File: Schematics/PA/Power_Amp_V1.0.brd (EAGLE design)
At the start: 46.7 x 73.3 mm, 99 parts, among them J1 4_PIN_AMPCONN, J11 SCREW_TERMINAL_4, J12 1725724, J13 1725724, J14 1725724, U1 LME49830, U2 LME49830, U3 LME49830

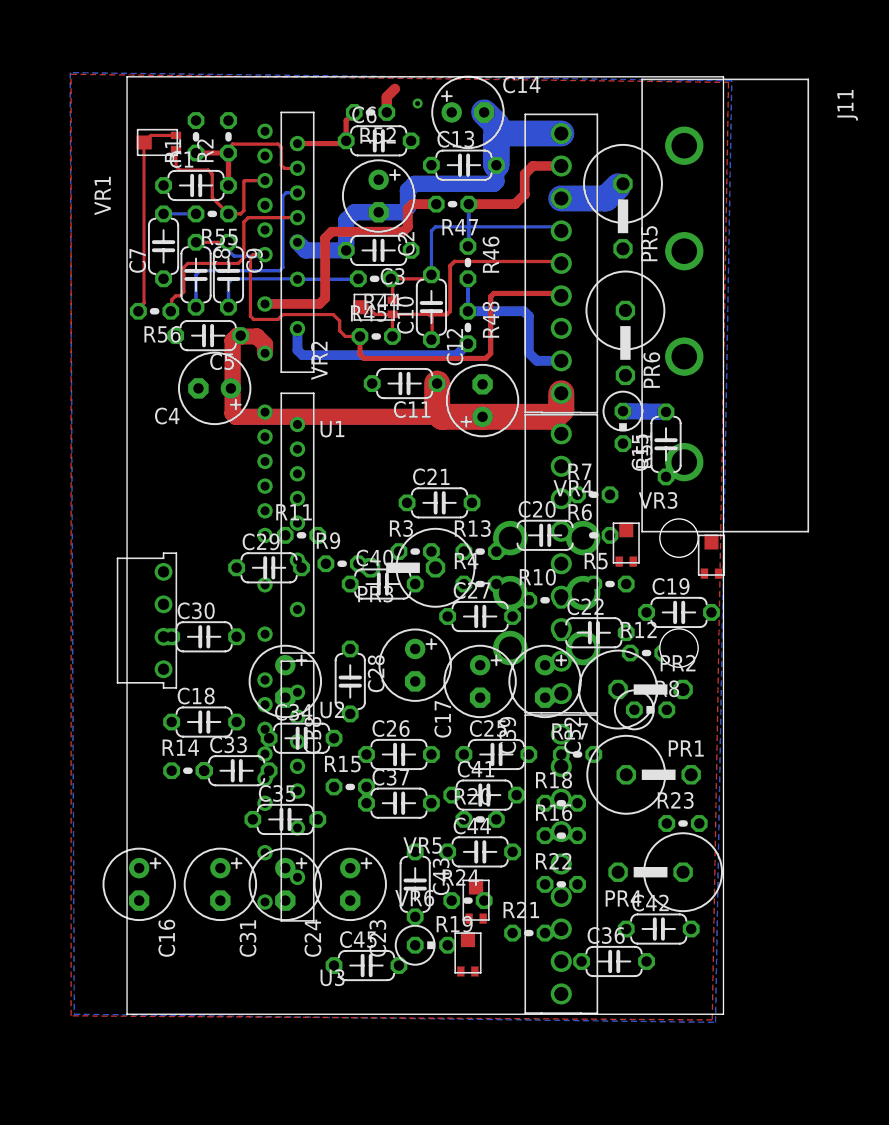
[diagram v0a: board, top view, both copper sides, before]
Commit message: Finished My PA and made changes to Carlos' PA
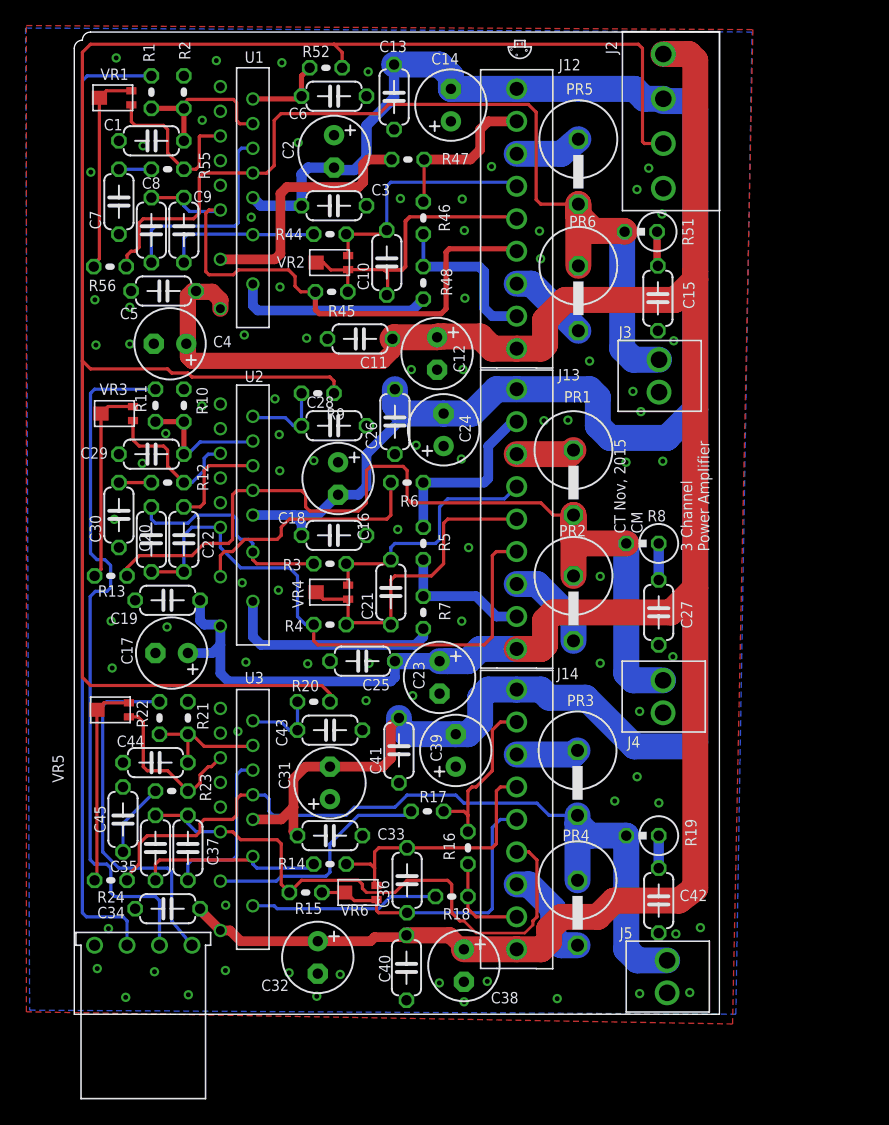
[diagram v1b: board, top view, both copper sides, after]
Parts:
- removed J11: SCREW_TERMINAL_4, Amplifier_Parts:SCREW_TERMINAL_4
- added J2: 1984633, Amplifier_Parts:1984633
- added J3, J4, J5: 2TERMINAL_SPEAKER, Amplifier_Parts:2TERMINAL_SPEAKER
- U$17: value MOLEX_6P -> (none); device Amplifier_Parts:MOLEX_6P -> PersonalLogos:MUSHROOM
- moved VR3 47.7 mm to (3.49, 47.0), turned to 90 degrees
- moved U$17 45.2 mm to (34.9, 75.4), turned to 180 degrees
- moved R23 40.1 mm to (7.62, 17.5), turned to 180 degrees
- moved C19 40.0 mm to (7.30, 32.4), turned to 180 degrees
- moved R12 39.8 mm to (7.30, 41.6), turned to 180 degrees
- moved C24 37.7 mm to (28.9, 45.7), turned to 90 degrees
- moved C16 35.4 mm to (20.6, 41.9)
- moved R22 34.0 mm to (6.67, 23.2), turned to 90 degrees
- moved C22 32.9 mm to (8.57, 37.1), turned to 90 degrees
- moved R10 32.1 mm to (8.57, 47.6), turned to 90 degrees
- moved VR5 32.1 mm to (3.17, 23.8), turned to 90 degrees
- moved R21 31.5 mm to (8.89, 23.2), turned to 90 degrees
- moved C20 30.8 mm to (6.03, 37.1), turned to 90 degrees
- moved C40 30.1 mm to (26.0, 3.64), turned to 270 degrees
- moved R13 29.0 mm to (2.86, 34.3), turned to 180 degrees
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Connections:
- net BASS renamed N$1
- net GND: now also J2.P$1, J3.P$2, J4.P$2, J5.P$2; no longer J11.1, U$17.P$2, U$17.P$4, U$17.P$6
- net MUTE: now also J2.P$2; no longer J11.2
- net N$12: now also J4.P$1; no longer U$17.P$3
- net N$75: now also J3.P$1; no longer U$17.P$1
- net N$77: now also J5.P$1; no longer U$17.P$5
- net V+: now also J2.P$4; no longer J11.4
- net V-: now also J2.P$3; no longer J11.3
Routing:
- net V+: track 42.0 -> 243.7 mm
- net V-: track 33.4 -> 195.3 mm
- net MUTE: track 2.10 -> 146.0 mm
- net RIGHT: track 0.00 -> 76.3 mm
- net N$12: track 0.00 -> 71.4 mm
- net N$75: track 16.2 -> 81.5 mm
- net N$77: track 0.00 -> 64.5 mm
- net N$1: track 0.00 -> 55.3 mm
- net L_VBE_E: track 0.00 -> 46.0 mm
- net B_VBE_E: track 0.00 -> 45.8 mm
- net LEFT: track 0.00 -> 28.4 mm
- net B_VBE_B: track 0.00 -> 25.4 mm
- net L_VBE_B: track 0.00 -> 23.2 mm
- net L_VBE_C: track 0.00 -> 20.7 mm
- net B_VBE_C: track 0.00 -> 19.6 mm
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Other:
- board size 46.7 x 73.3 mm -> 50.5 x 76.8 mm
- board text added: "3 Channel Power Amplifier"
- board text added: "CT Nov, 2015 CM"
